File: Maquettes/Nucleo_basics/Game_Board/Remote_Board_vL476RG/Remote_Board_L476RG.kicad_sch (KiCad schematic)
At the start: 43 parts, among them CON1 MikroE-nRF-S-module, J1 LCD_SD, J10 3.3V_reg, J2 JoyStick, J3 AnalogIn, J4 BAT_IN, J5 Morpho_Gauche, J6 Morpho_Droite, J7 I2C_Visu, J8 I2C_EXT, J9 GND_reg, SW1 SW_1, SW2 SW_2, SW3 SW_3, SW4 SW_4, SW5 SW_5, U1 MCP23008-xP

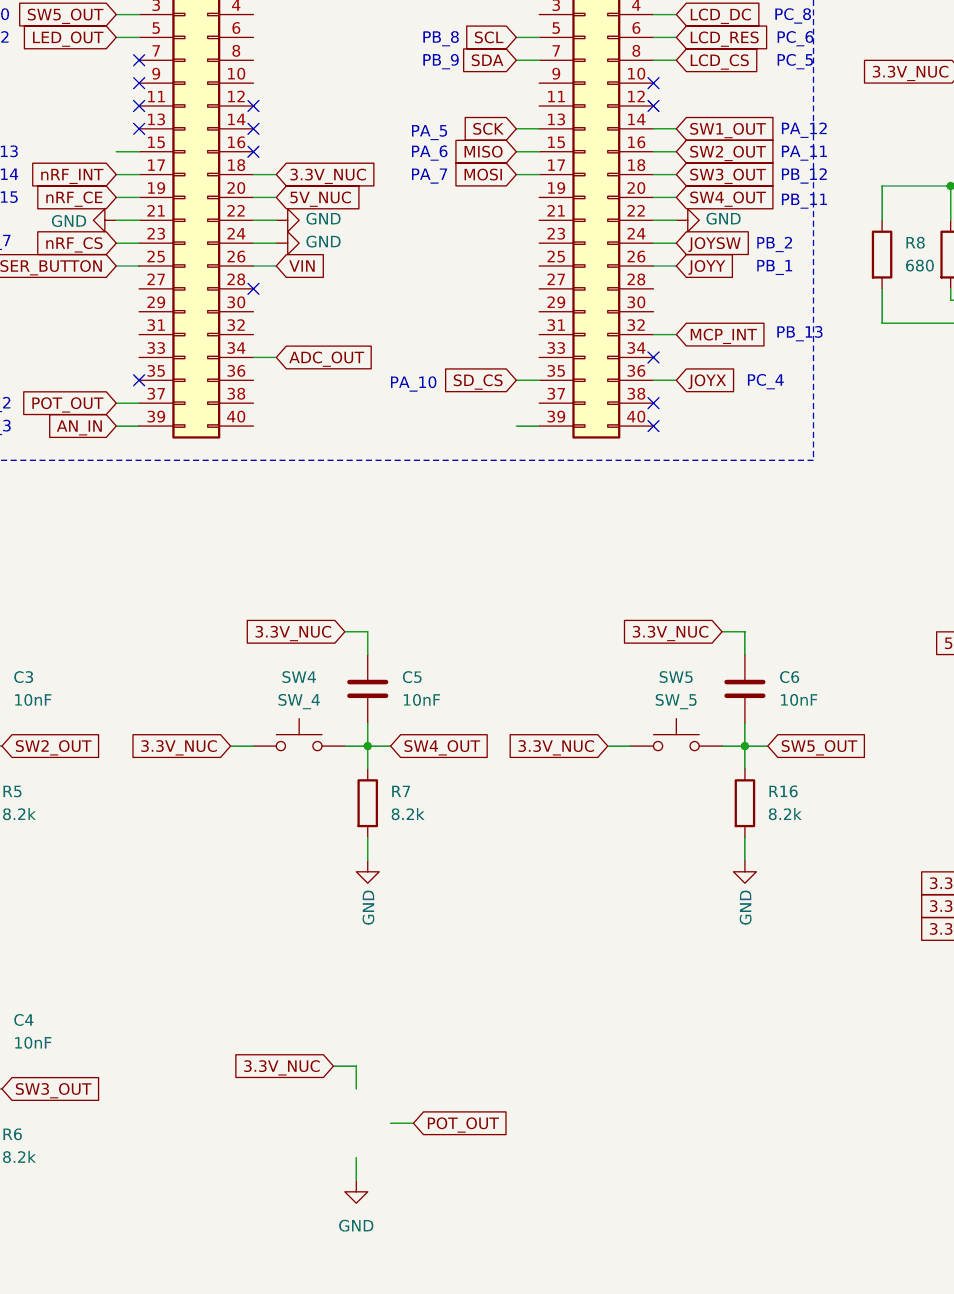
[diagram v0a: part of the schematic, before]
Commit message: Update Boards
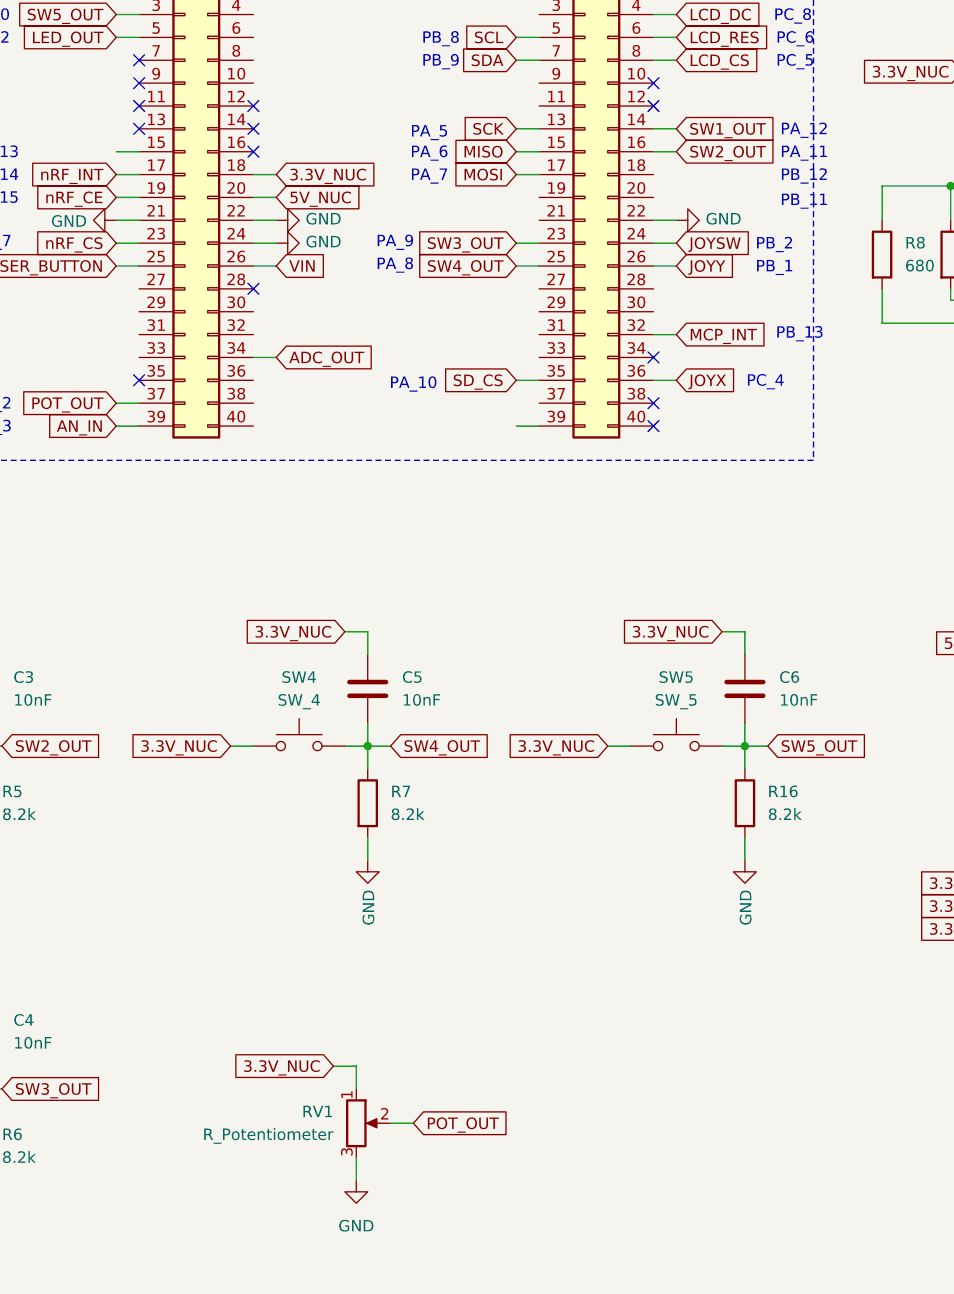
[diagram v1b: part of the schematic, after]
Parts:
- added RV1: R_Potentiometer, Potentiometer_THT:Potentiometer_Vishay_T73YP_Vertical, symbol Device:R_Potentiometer
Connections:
- net 3.3V_NUC: now also RV1.1
- net GND: now also RV1.3
- net POT_OUT: now also RV1.2
- net SW3_OUT: now also J6.23 (Pin_23); no longer J6.18 (Pin_18)
- net SW4_OUT: now also J6.25 (Pin_25); no longer J6.20 (Pin_20)
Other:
- note added: "PA_8"
- note added: "PA_9"
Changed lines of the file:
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@@
 	(wire
 		(pts
+			(xy 140.97 81.28) (xy 143.51 81.28)
+		)
+		(stroke
+			(width 0)
+			(type default)
+		)
+	)
+	(wire
+		(pts
 			(xy 247.65 55.88) (xy 250.19 55.88)
 		)
@@
 	(wire
 		(pts
-			(xy 156.21 73.66) (xy 158.75 73.66)
-		)
-		(stroke
-			(width 0)
-			(type default)
-		)
-	)
-	(wire
-		(pts
 			(xy 163.83 124.46) (xy 166.37 124.46)
 		)
@@
 	(wire
 		(pts
-			(xy 271.78 161.29) (xy 274.32 161.29)
+			(xy 140.97 83.82) (xy 143.51 83.82)
 		)
 		(stroke
@@
 	(wire
 		(pts
-			(xy 199.39 152.4) (xy 196.85 152.4)
+			(xy 271.78 161.29) (xy 274.32 161.29)
 		)
 		(stroke
@@
 	(wire
 		(pts
-			(xy 156.21 76.2) (xy 158.75 76.2)
+			(xy 199.39 152.4) (xy 196.85 152.4)
 		)
 		(stroke
@@
 		)
 	)
+	(text "PA_9"
+		(exclude_from_sim no)
+		(at 127.508 81.28 0)
+		(effects
+			(font
+				(size 1.27 1.27)
+			)
+		)
+	)
 	(text "PC_5"
 		(exclude_from_sim no)
@@
 		)
 	)
+	(text "PA_8"
+		(exclude_from_sim no)
+		(at 127.508 83.82 0)
+		(effects
+			(font
+				(size 1.27 1.27)
+			)
+		)
+	)
 	(text "PA_10"
 		(exclude_from_sim no)
@@
 	(global_label "SW3_OUT"
 		(shape input)
-		(at 158.75 73.66 0)
+		(at 140.97 81.28 180)
 		(effects
 			(font
 				(size 1.27 1.27)
 			)
-			(justify left)
+			(justify right)
 		)
 		(property "Intersheetrefs" "${INTERSHEET_REFS}"
-			(at 158.75 73.66 0)
+			(at 140.97 81.28 0)
 			(effects
 				(font
@@
 	(global_label "SW4_OUT"
 		(shape input)
-		(at 158.75 76.2 0)
+		(at 140.97 83.82 180)
 		(effects
 			(font
 				(size 1.27 1.27)
 			)
-			(justify left)
+			(justify right)
 		)
 		(property "Intersheetrefs" "${INTERSHEET_REFS}"
-			(at 158.75 76.2 0)
+			(at 140.97 83.82 0)
 			(effects
 				(font
@@
 					(unit 1)
 				)
+			)
+		)
+	)
+	(symbol
+		(lib_id "Device:R_Potentiometer")
+		(at 123.19 179.07 0)
+		(unit 1)
+		(exclude_from_sim no)
+		(in_bom yes)
+		(on_board yes)
+		(dnp no)
+		(fields_autoplaced yes)
+		(property "Reference" "RV1"
+			(at 120.65 177.7999 0)
+			(effects
+				(font
+					(size 1.27 1.27)
+				)
+				(justify right)
+			)
+		)
+		(property "Value" "R_Potentiometer"
+			(at 120.65 180.3399 0)
+			(effects
+				(font
+					(size 1.27 1.27)
+				)
+				(justify right)
+			)
+		)
+		(property "Footprint" "Potentiometer_THT:Potentiometer_Vishay_T73YP_Vertical"
+			(at 123.19 179.07 0)
+			(effects
+				(font
+					(size 1.27 1.27)
+				)
+				(hide yes)
+			)
+		)
+		(property "Datasheet" "~"
+			(at 123.19 179.07 0)
+			(effects
+				(font
+					(size 1.27 1.27)
+				)
+				(hide yes)
+			)
+		)
+		(property "Description" "Potentiometer"
+			(at 123.19 179.07 0)
+			(effects
+				(font
+					(size 1.27 1.27)
+				)
+				(hide yes)
+			)
+		)
+		(pin "1"
+		)
+		(pin "2"
+		)
+		(pin "3"
+		)
+		(instances
+			(project "Remote_Board_L476RG"
+				(path "/44ad8000-4ee7-4966-8fe6-195894dfb602"
+					(reference "RV1")
+					(unit 1)
+				)
